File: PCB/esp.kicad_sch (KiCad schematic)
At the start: 45 parts, among them J1 USB_C_Receptacle_USB2.0_14P, J2 Conn_01x04_Pin, SW1 RESET, SW2 BOOT, U1 ESP32-C3, U2 W25Q128JVP, U3 USBLC6-2P6, U4 MS5611-01BA, U5 SPX3819M5-L-3-3, U6 SHTC3, Y2 Crystal_GND24

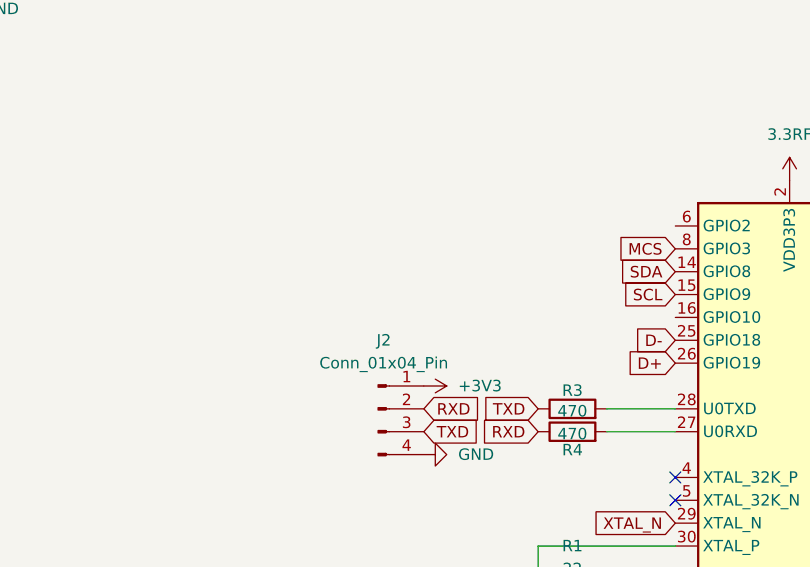
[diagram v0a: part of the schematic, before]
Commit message: SD
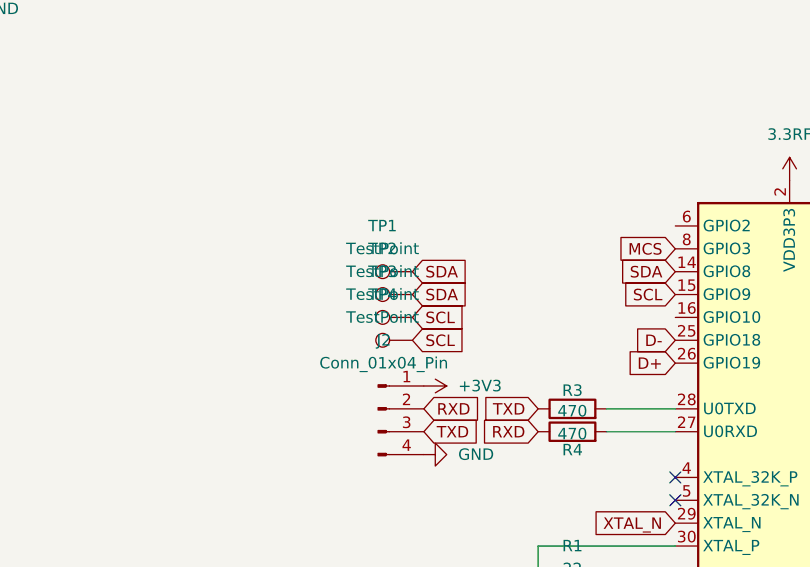
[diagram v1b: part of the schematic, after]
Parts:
- added TP1, TP2, TP3, TP4: TestPoint, Connector_PinHeader_1.00mm:PinHeader_1x01_P1.00mm_Vertical, symbol Connector:TestPoint
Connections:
- net SCL: now also TP3.1, TP4.1
- net SDA: now also TP1.1, TP2.1
